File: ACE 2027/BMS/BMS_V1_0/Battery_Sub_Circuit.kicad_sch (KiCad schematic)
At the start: 12 parts, among them Q1 NTR2101P, Q2 NPN, SW1 E-STOP, SW2 RESET_SWITCH

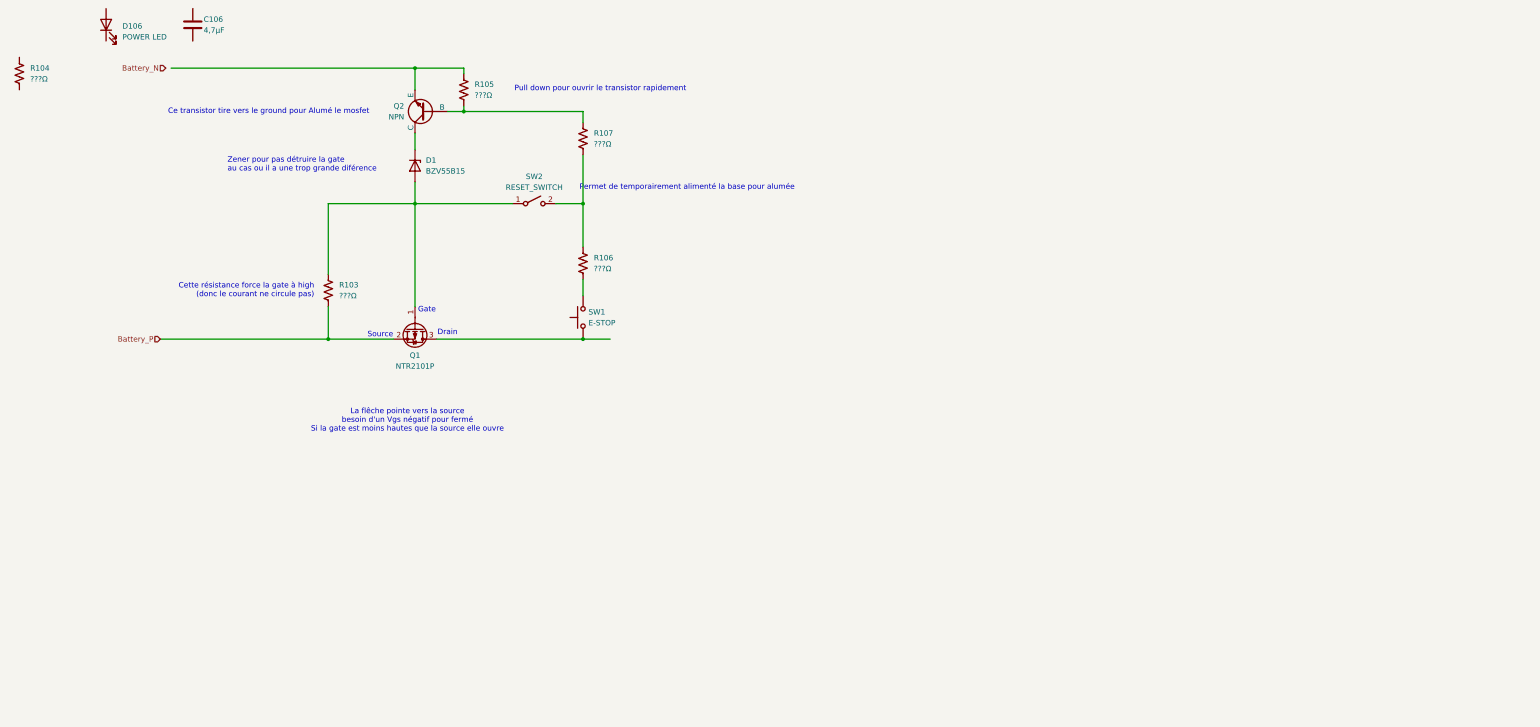
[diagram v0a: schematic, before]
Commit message: Avancement circuit de sécurité
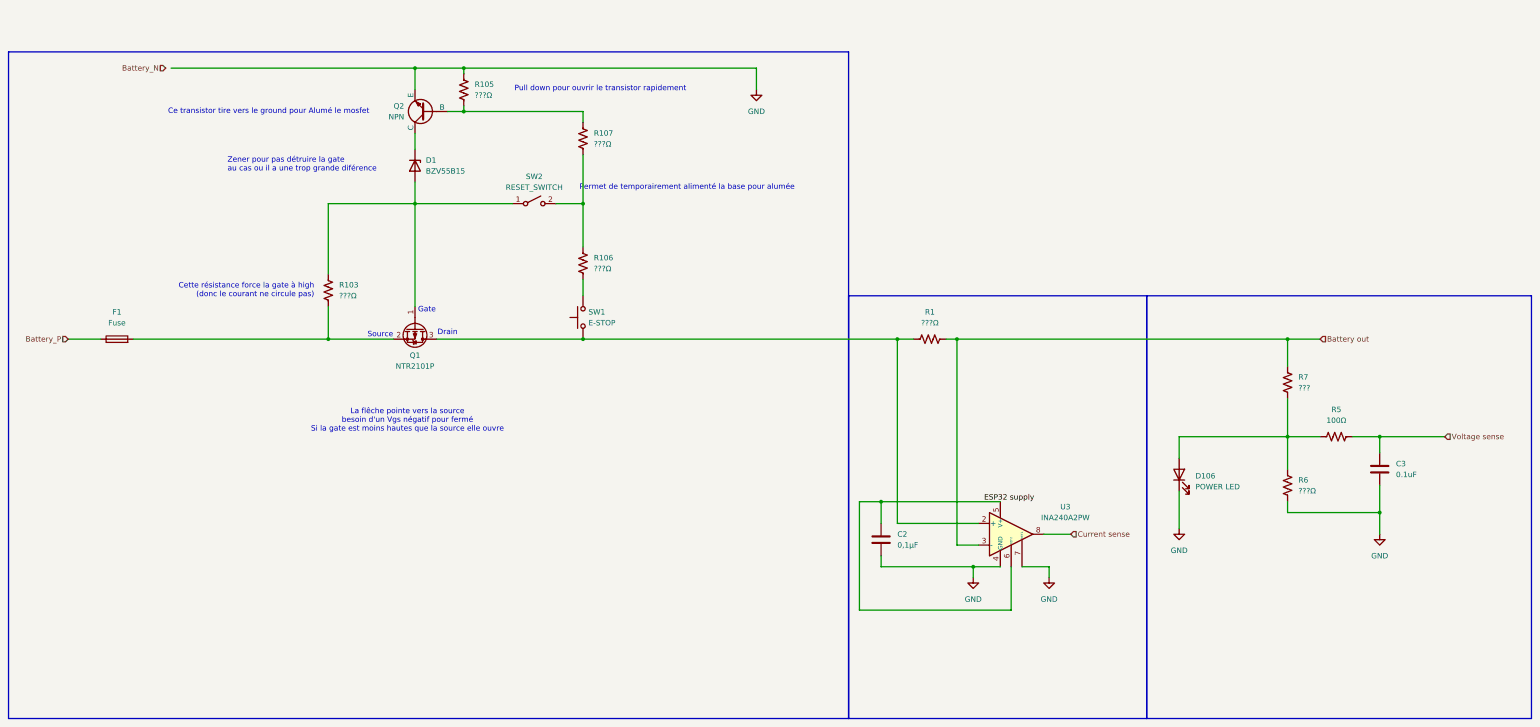
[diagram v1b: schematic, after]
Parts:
- removed C106: 4,7µF, Capacitor_SMD:C_0805_2012Metric_Pad1.18x1.45mm_HandSolder, symbol Device:C
- removed R104: ???Ω, Resistor_SMD:R_0805_2012Metric_Pad1.20x1.40mm_HandSolder, symbol Device:R_US
- added C2: 0,1µF, Capacitor_SMD:C_0805_2012Metric, symbol Device:C
- added C3: 0.1uF, Capacitor_SMD:C_0805_2012Metric, symbol Device:C
- added F1: Fuse, symbol Device:Fuse
- added R1: ???Ω, Resistor_SMD:R_2512_6332Metric_Pad1.40x3.35mm_HandSolder, symbol Device:R_US
- added R5: 100Ω, Resistor_SMD:R_0805_2012Metric, symbol Device:R_US
- added R6: ???Ω, Resistor_SMD:R_0805_2012Metric, symbol Device:R_US
- added R7: ???, Resistor_SMD:R_0805_2012Metric, symbol Device:R_US
- added U3: INA240A2PW, Package_SO:TSSOP-8_4.4x3mm_P0.65mm, symbol Amplifier_Current:INA240A2PW
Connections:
- net Battery_P: now also F1.1; no longer Q1.2 (S), R103.2
- net at Q1.3 (D), SW1.1: now also R1.1, U3.2 (+)
- net GND: now reaches Q2.3 (E), R105.1
- net GND: now also D106.1 (K), C2.2, C3.2, R6.1, U3.1 (GND), U3.4 (GND), U3.7 (REF1)
- net at D106.2 (A): now also R5.2, R6.2, R7.1
- new net: F1.2, Q1.2 (S), R103.2
- new net Battery out: R1.2, R7.2, U3.3 (-)
- new net Current sense: U3.8
- new net ESP32 supply: C2.1, U3.5 (V+), U3.6 (REF2)
- new net Voltage sense: C3.1, R5.1
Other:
- moved on the sheet: D106
